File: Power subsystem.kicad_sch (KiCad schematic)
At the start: 33 parts, among them J1 Conn_01x02_Pin, J2 Conn_01x04_Pin, J3 Connector, USB-TYPE-C-16P, Q1 AO3401A, Q2 MMBT5551 200-300, Q3 MMBT5401 200-300, SW1 SW_SPST, U1 INA219AxD, U2 CH224K, U5 TP4056-42-ESOP8

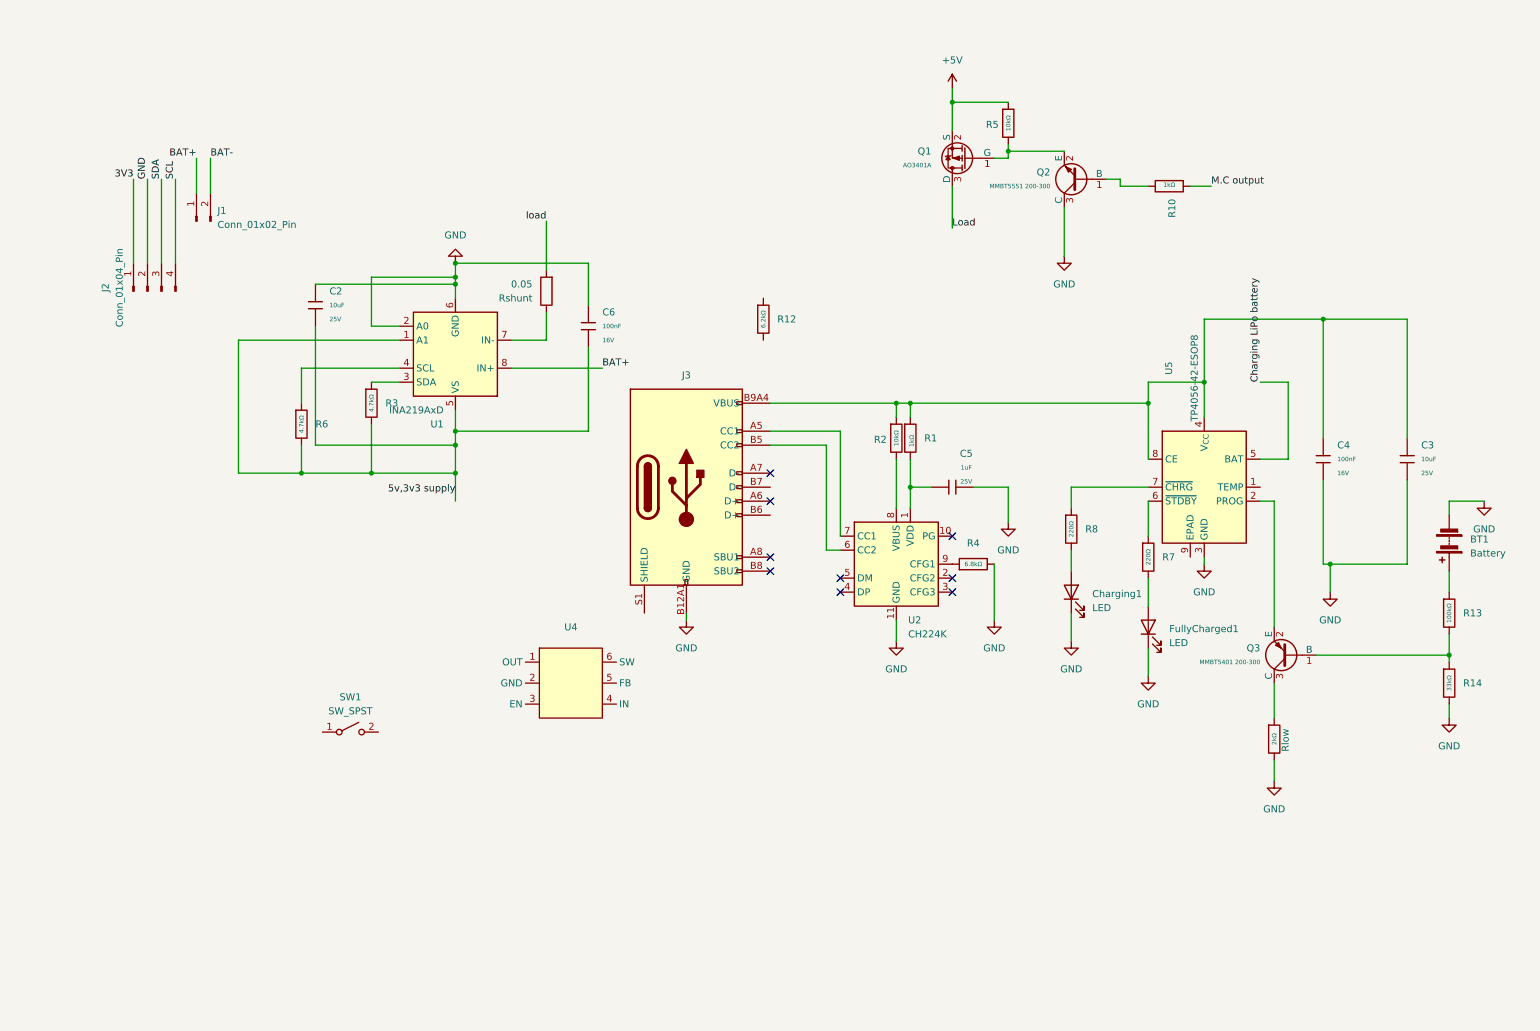
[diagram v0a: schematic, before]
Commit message: Add files via upload
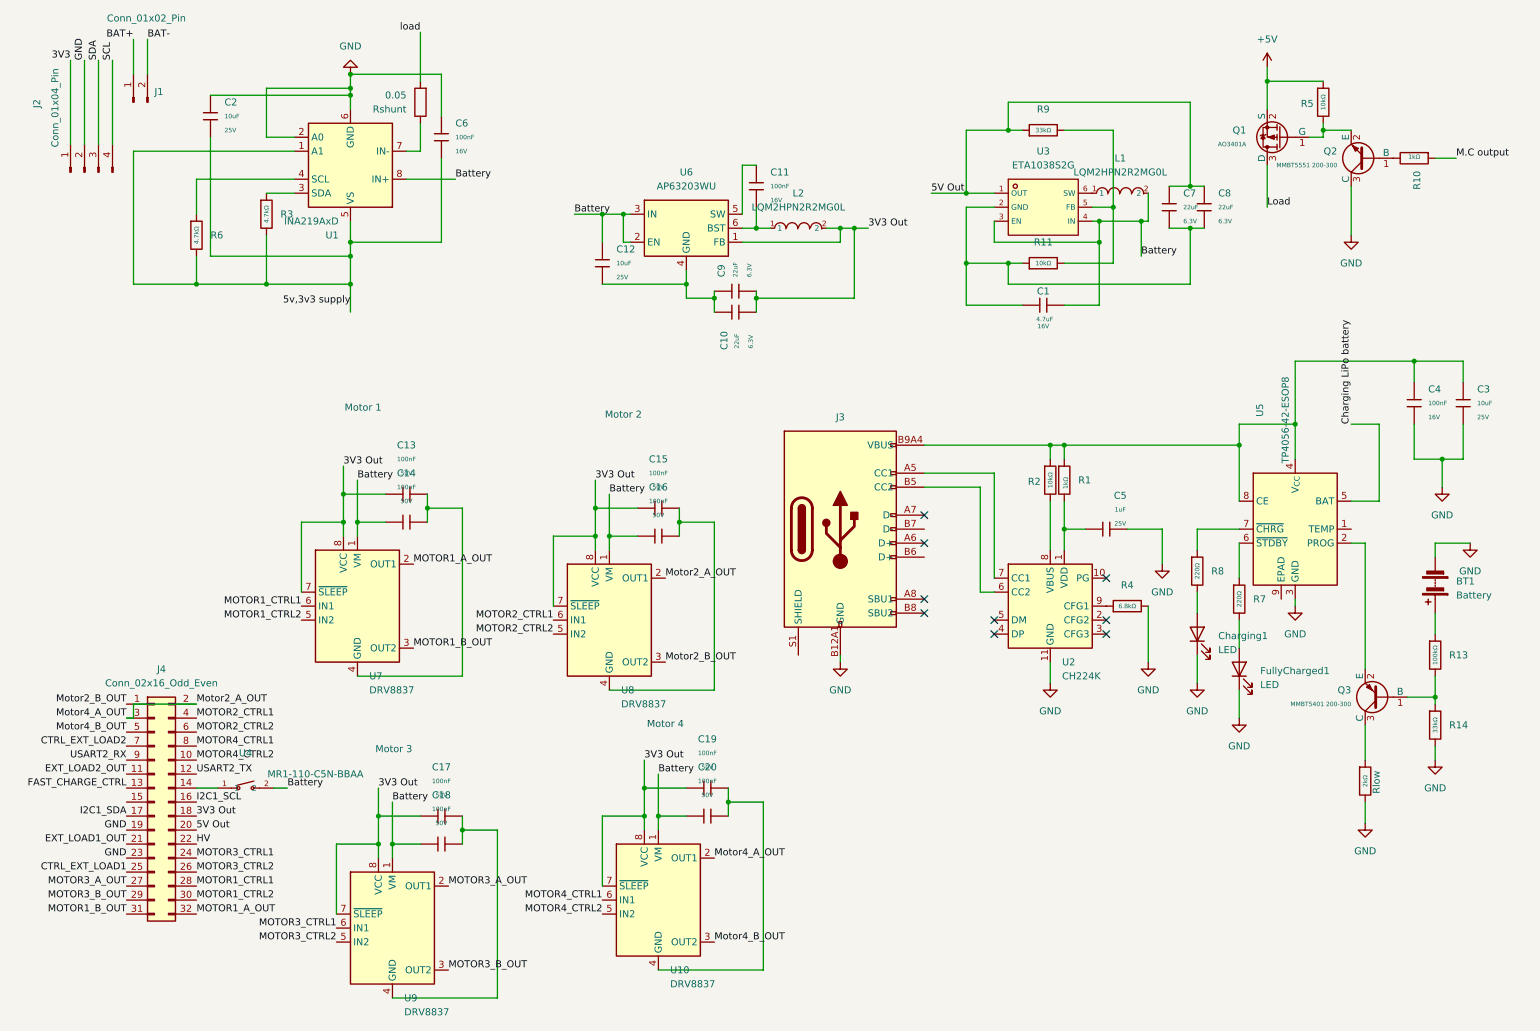
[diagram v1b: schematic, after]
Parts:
- removed R12: 6.2kΩ, PCM_JLCPCB:R_0603, symbol PCM_JLCPCB-Resistors:0603,6.2kΩ
- removed SW1: SW_SPST, symbol Switch:SW_SPST
- removed U4: ~, ETA1038:Untitled, symbol ETA1038:ETA1038
- added C1: 4.7uF, PCM_JLCPCB:C_0603, symbol PCM_JLCPCB-Capacitors:0603,4.7uF
- added C10, C7, C8, C9: 22uF, PCM_JLCPCB:C_0603, symbol PCM_JLCPCB-Capacitors:0603,22uF
- added C11: 100nF, PCM_JLCPCB:C_0402, symbol PCM_JLCPCB-Capacitors:0402,100nF
- added C12: 10uF, PCM_JLCPCB:C_0805, symbol PCM_JLCPCB-Capacitors:0805,10uF
- added C13, C14, C15, C16, C17, C18, C19, C20: 100nF, PCM_JLCPCB:C_0603, symbol PCM_JLCPCB-Capacitors:0603,100nF
- added J4: Conn_02x16_Odd_Even, Connector_PinHeader_2.54mm:PinHeader_2x16_P2.54mm_Vertical, symbol Connector_Generic:Conn_02x16_Odd_Even
- added L1, L2: LQM2HPN2R2MG0L, myparts:L1008, symbol myparts:LQM2HPN2R2MG0L
- added R11: 10kΩ, PCM_JLCPCB:R_0603, symbol PCM_JLCPCB-Resistors:0603,10kΩ
- added R9: 33kΩ, PCM_JLCPCB:R_0603, symbol PCM_JLCPCB-Resistors:0603,33kΩ
- added U10, U7, U8, U9: DRV8837, Package_SON:WSON-8-1EP_2x2mm_P0.5mm_EP0.9x1.6mm, symbol Driver_Motor:DRV8837
- added U3: ETA1038S2G, myparts:SOT-23-6_L2.9-W1.6-P0.95-LS2.8-BR, symbol myparts:ETA1038S2G
- added U4: MR1-110-C5N-BBAA, myparts:SW-TH_MR1-110-C5N-BBAA, symbol myparts:MR1-110-C5N-BBAA
- added U6: AP63203WU, Package_TO_SOT_SMD:TSOT-23-6, symbol Regulator_Switching:AP63203WU
- J1: footprint (none) -> Connector_JST:JST_PH_B2B-PH-K_1x02_P2.00mm_Vertical
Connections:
- net BAT+: no longer U1.8 (IN+)
- net GND: now also J4.19 (Pin_19), J4.23 (Pin_23)
- new net: R11.2, R9.2, U3.5 (FB)
- new net: C1.1, C7.2, C8.2, R11.1, U3.2 (GND)
- new net: L1.1, U3.6 (SW)
- new net: C11.2, L2.1, U6.6 (BST)
- new net: C10.1, C12.2, C9.1, U6.4 (GND)
- new net: C17.2, C18.2, U9.4 (GND), U9.9 (GND)
- new net: C15.2, C16.2, U8.4 (GND), U8.9 (GND)
- new net: C19.2, C20.2, U10.4 (GND), U10.9 (GND)
- new net: C13.2, C14.2, U7.4 (GND), U7.9 (GND)
- new net: C11.1, U6.5 (SW)
- new net: J4.14 (Pin_14), U4.1
- new net 3V3 Out: C10.2, C13.1, C15.1, C17.1, C19.1, C9.2, J4.18 (Pin_18), L2.2, U10.7 (~{SLEEP}), U10.8 (VCC), U6.1 (FB), U7.7 (~{SLEEP}), U7.8 (VCC), U8.7 (~{SLEEP}), U8.8 (VCC), U9.7 (~{SLEEP}), U9.8 (VCC)
- new net 5V Out: C7.1, C8.1, J4.20 (Pin_20), R9.1, U3.1 (OUT)
- new net Battery: C1.2, C12.1, C14.1, C16.1, C18.1, C20.1, L1.2, U1.8 (IN+), U10.1 (VM), U3.3 (EN), U3.4 (IN), U4.2, U6.2 (EN), U6.3 (IN), U7.1 (VM), U8.1 (VM), U9.1 (VM)
- new net CTRL_EXT_LOAD1: J4.25 (Pin_25)
- new net CTRL_EXT_LOAD2: J4.7 (Pin_7)
- new net EXT_LOAD1_OUT: J4.21 (Pin_21)
- new net EXT_LOAD2_OUT: J4.11 (Pin_11)
- new net FAST_CHARGE_CTRL: J4.13 (Pin_13)
- new net HV: J4.22 (Pin_22)
- new net I2C1_SCL: J4.16 (Pin_16)
- new net I2C1_SDA: J4.17 (Pin_17)
- new net MOTOR1_A_OUT: J4.32 (Pin_32), U7.2 (OUT1)
- new net MOTOR1_B_OUT: J4.31 (Pin_31), U7.3 (OUT2)
- new net MOTOR1_CTRL1: J4.28 (Pin_28), U7.6 (IN1)
- new net MOTOR1_CTRL2: J4.30 (Pin_30), U7.5 (IN2)
- new net MOTOR2_CTRL1: J4.4 (Pin_4), U8.6 (IN1)
- new net MOTOR2_CTRL2: J4.6 (Pin_6), U8.5 (IN2)
- new net MOTOR3_A_OUT: J4.27 (Pin_27), U9.2 (OUT1)
- new net MOTOR3_B_OUT: J4.29 (Pin_29), U9.3 (OUT2)
- new net MOTOR3_CTRL1: J4.24 (Pin_24), U9.6 (IN1)
- new net MOTOR3_CTRL2: J4.26 (Pin_26), U9.5 (IN2)
- new net MOTOR4_CTRL1: J4.8 (Pin_8), U10.6 (IN1)
- new net MOTOR4_CTRL2: J4.10 (Pin_10), U10.5 (IN2)
- new net Motor2_A_OUT: J4.2 (Pin_2), J4.3 (Pin_3), U10.2 (OUT1), U8.2 (OUT1)
- new net Motor2_B_OUT: J4.1 (Pin_1), U8.3 (OUT2)
- new net Motor4_B_OUT: J4.5 (Pin_5), U10.3 (OUT2)
- new net USART2_RX: J4.9 (Pin_9)
- new net USART2_TX: J4.12 (Pin_12)
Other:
- note added: "Motor 1"
- note added: "Motor 2"
- note added: "Motor 3"
- note added: "Motor 4"
- moved on the sheet: BT1, C2, C3, C4, C5, C6, Charging1, FullyCharged1, J1, J2, J3, Q1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
